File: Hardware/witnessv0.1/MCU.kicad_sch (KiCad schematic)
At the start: 8 parts, among them J1 Conn_01x02, U1 RP2354B

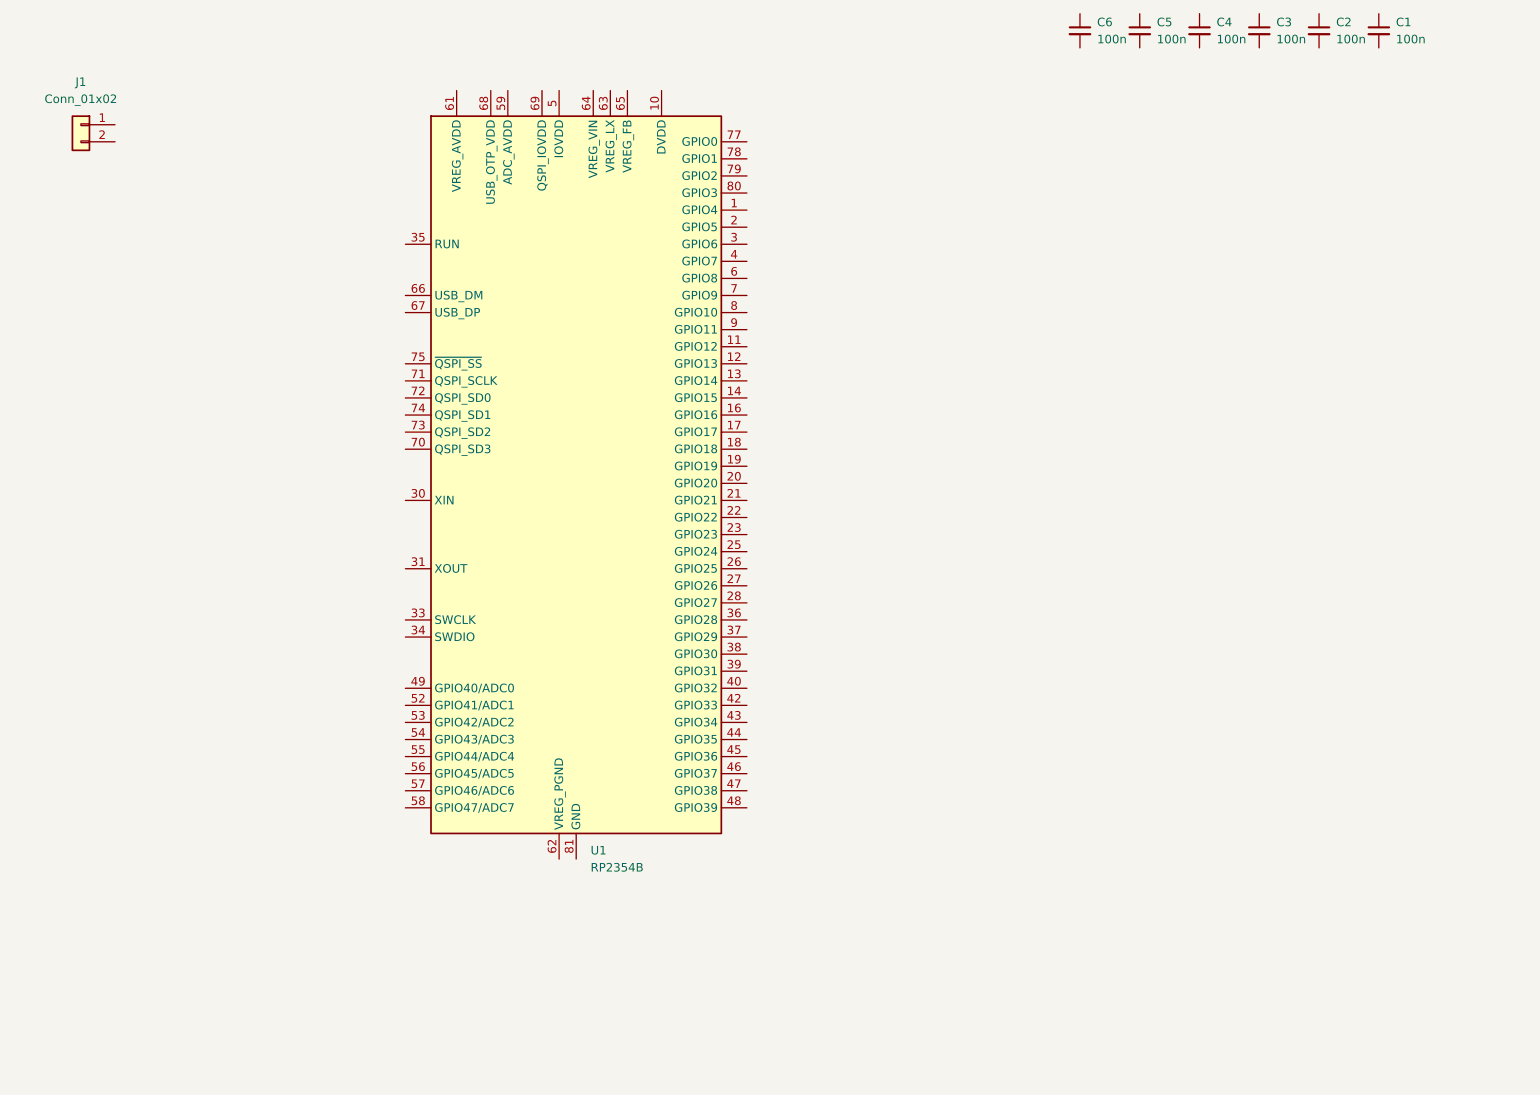
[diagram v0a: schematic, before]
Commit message: esp32 mcu
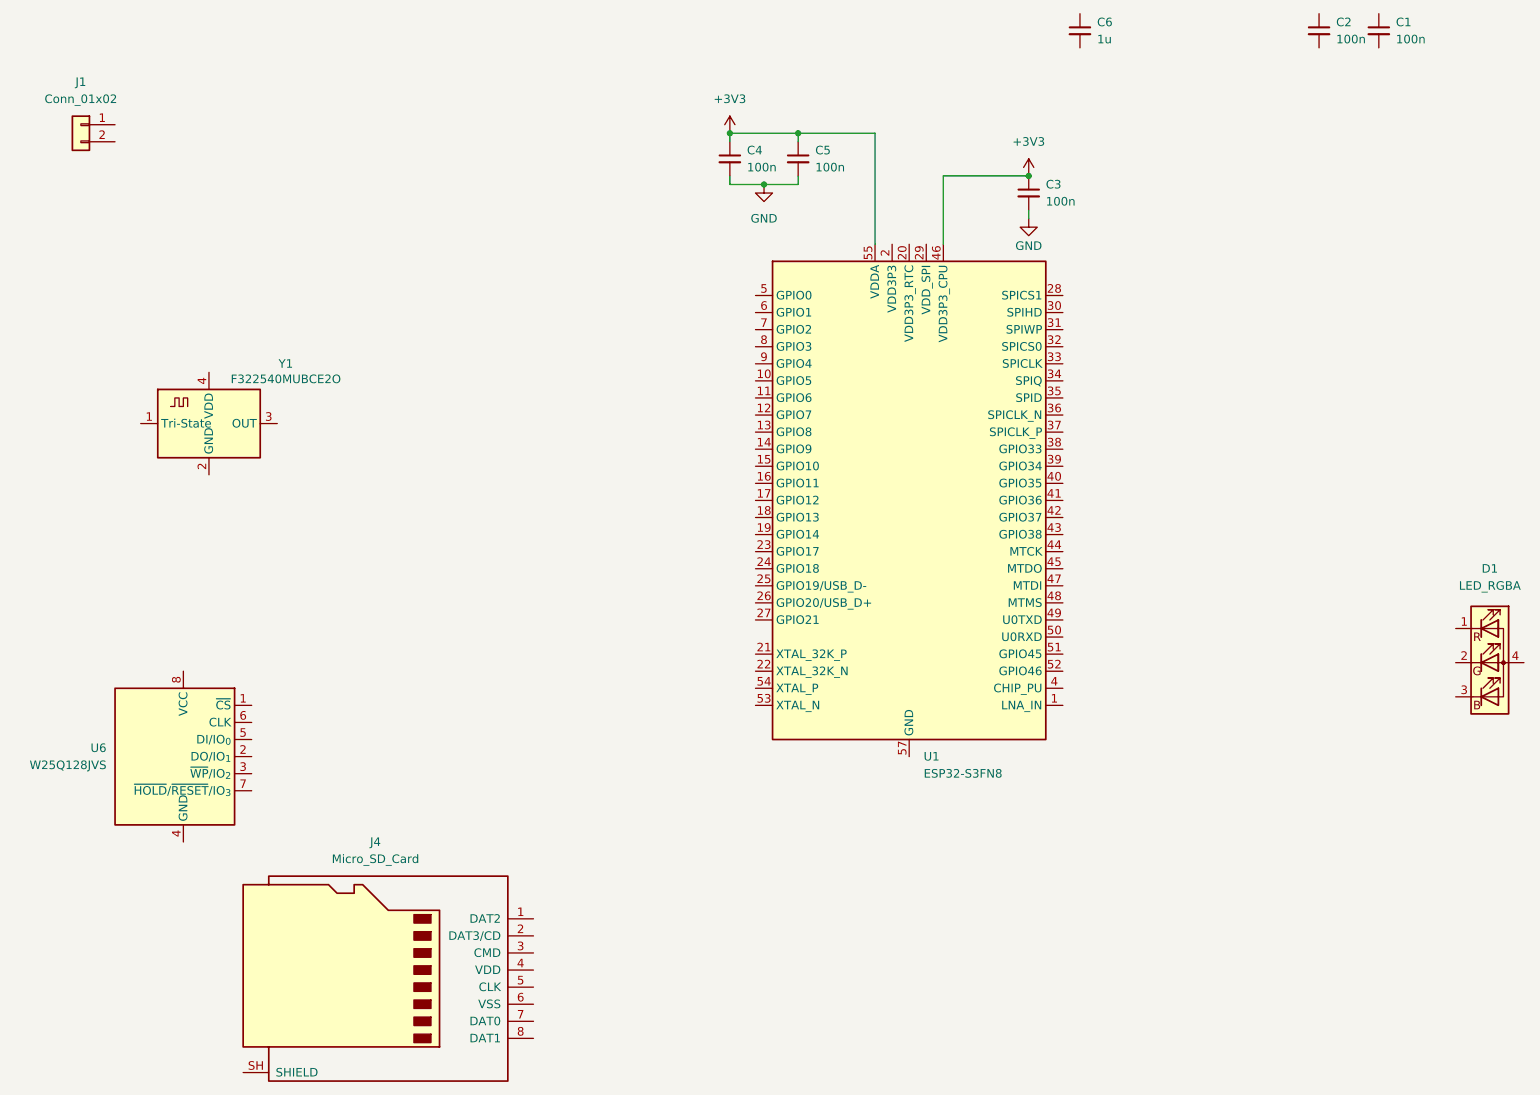
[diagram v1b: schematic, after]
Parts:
- removed U1: RP2354B, Package_DFN_QFN:QFN-80-1EP_10x10mm_P0.4mm_EP3.4x3.4mm, symbol MCU_RaspberryPi:RP2354B
- added D1: LED_RGBA, symbol Device:LED_RGBA
- added J4: Micro_SD_Card, Connector_Card:microSD_HC_Wuerth_693072010801, symbol Connector:Micro_SD_Card
- added U1: ESP32-S3FN8, Package_DFN_QFN:QFN-56-1EP_7x7mm_P0.4mm_EP4x4mm, symbol MCU_Espressif:ESP32-S3
- added U6: W25Q128JVS, Package_SO:SOIC-8_5.3x5.3mm_P1.27mm, symbol Memory_Flash:W25Q128JVS
- added Y1: F322540MUBCE2O, Crystal:Crystal_SMD_3225-4Pin_3.2x2.5mm, symbol Oscillator:ASCO
- C6: value 100n -> 1u
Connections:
- net +3V3: now reaches C5.1
- net +3V3: now also C3.1, C4.1, U1.46 (VDD3P3_CPU), U1.55 (VDDA), U1.56 (VDDA)
- net GND: now reaches C5.2
- net GND: now also C3.2, C4.2
- new net: U1.2 (VDD3P3), U1.3 (VDD3P3)
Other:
- moved on the sheet: C3, C4, C5
